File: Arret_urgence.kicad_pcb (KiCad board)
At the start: 2 copper layers, 30 x 22 mm, 7 parts, among them J1 Conn_01x02, J2 USB_C_Receptacle_USB2.0, J3 USB_C_Receptacle_USB2.0

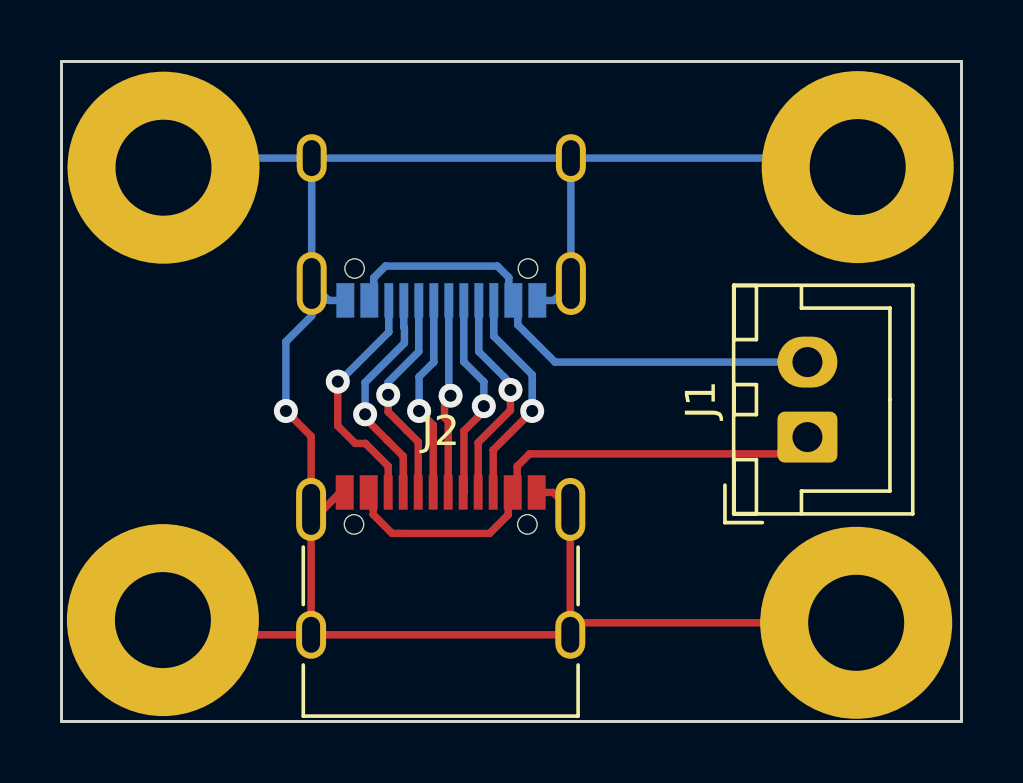
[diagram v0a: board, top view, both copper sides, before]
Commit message: modif schematic
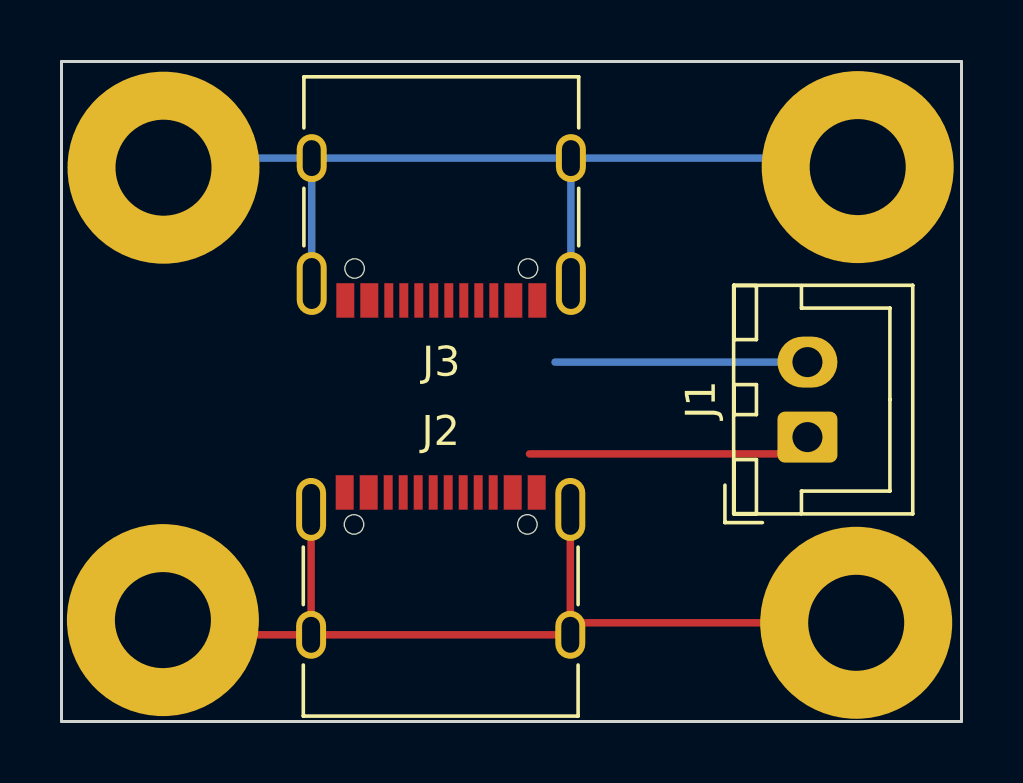
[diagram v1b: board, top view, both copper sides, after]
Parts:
- J3: moved to F.Cu
- turned J3 to 180 degrees
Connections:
- J3 pad A5: Net-(J2-PadA5) -> Net-(J2-PadB5)
- J3 pad A6: Net-(J2-PadA6) -> Net-(J2-PadB6)
- J3 pad A7: Net-(J2-PadA7) -> Net-(J2-PadB7)
- J3 pad A8: Net-(J2-PadA8) -> Net-(J2-PadB8)
- J3 pad B5: Net-(J2-PadB5) -> Net-(J2-PadA5)
- J3 pad B6: Net-(J2-PadB6) -> Net-(J2-PadA6)
- J3 pad B7: Net-(J2-PadB7) -> Net-(J2-PadA7)
- J3 pad B8: Net-(J2-PadB8) -> Net-(J2-PadA8)
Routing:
- net +5V: track 36.0 -> 17.9 mm
- net GND: track 77.8 -> 63.6 mm, vias 1 -> 0
- net Net-(J2-PadB8): track 8.03 -> 0.00 mm, vias 1 -> 0
- net Net-(J2-PadA5): track 7.48 -> 0.00 mm, vias 1 -> 0
- net Net-(J2-PadB5): track 7.47 -> 0.00 mm, vias 1 -> 0
- net Net-(J2-PadA8): track 7.28 -> 0.00 mm, vias 1 -> 0
- net Net-(J2-PadB7): track 7.24 -> 0.00 mm, vias 1 -> 0
- net Net-(J2-PadB6): track 6.97 -> 0.00 mm, vias 1 -> 0
- net Net-(J2-PadA6): track 6.80 -> 0.00 mm, vias 1 -> 0
- net Net-(J2-PadA7): track 6.56 -> 0.00 mm, vias 1 -> 0
